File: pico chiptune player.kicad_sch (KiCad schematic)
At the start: 35 parts, among them J2 MicroSD, SW1 Play / Pause, SW2 Next, SW3 Previous, U1 AY-3-8910, U2 0.96"OLED_I2C, U3 PAM8302, U4 YM2149F, U5 PAM8302

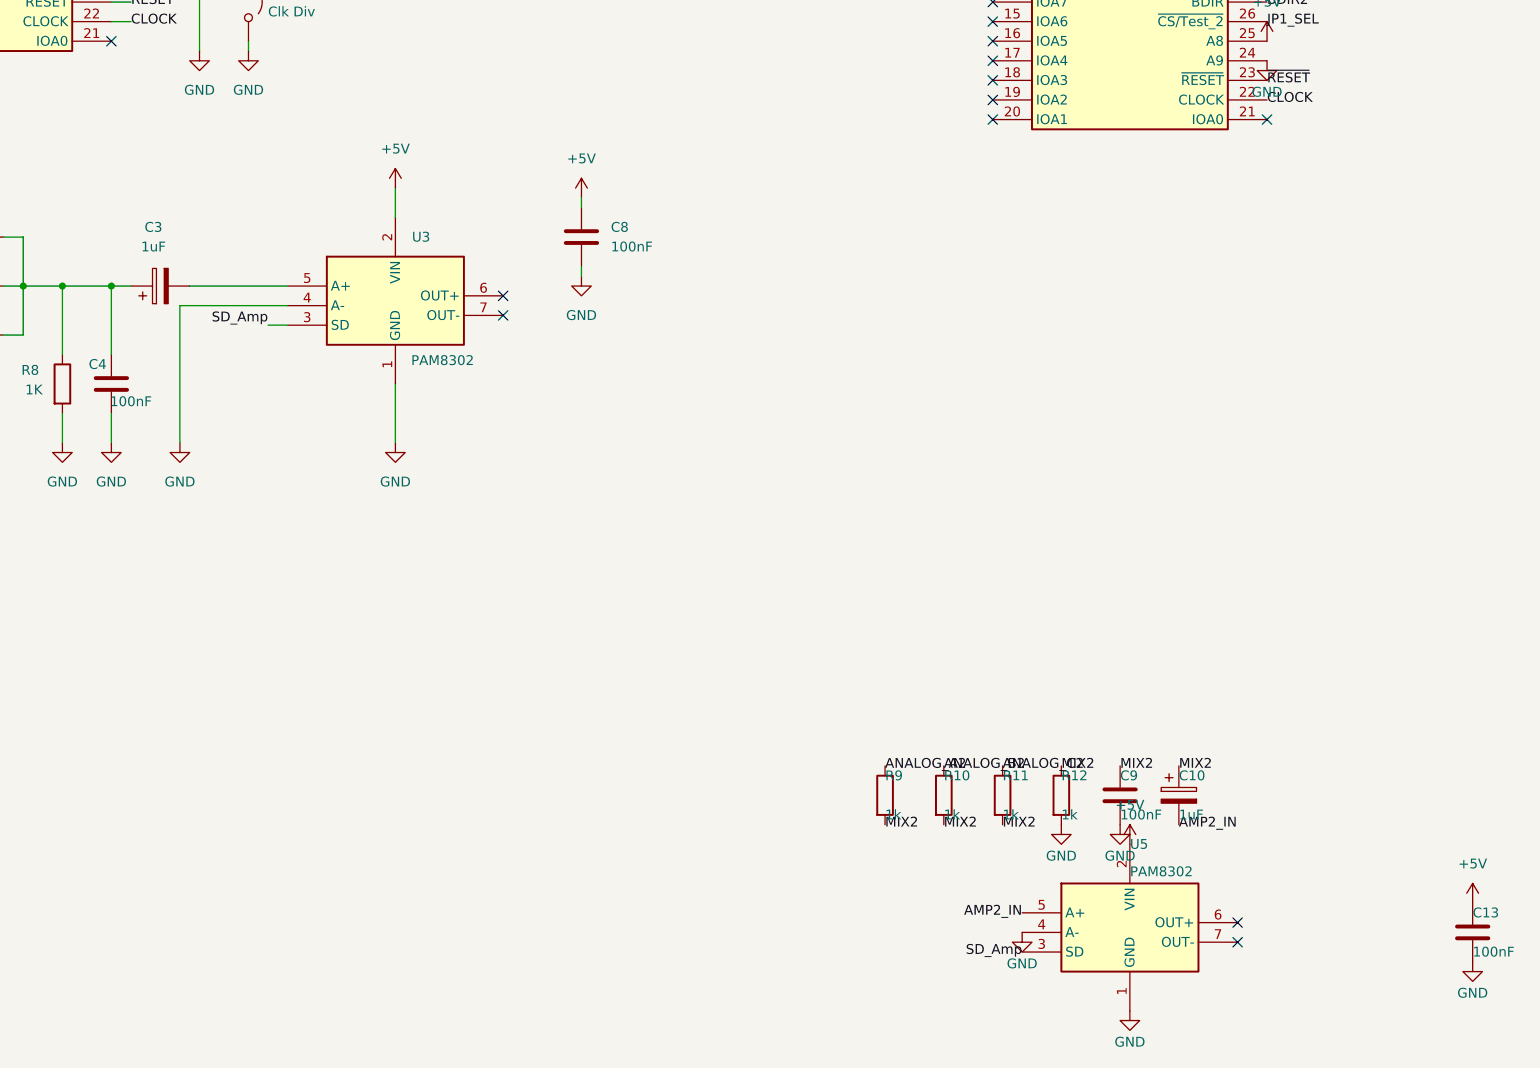
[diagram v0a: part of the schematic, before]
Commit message: Refactor code structure for improved readability and maintainability
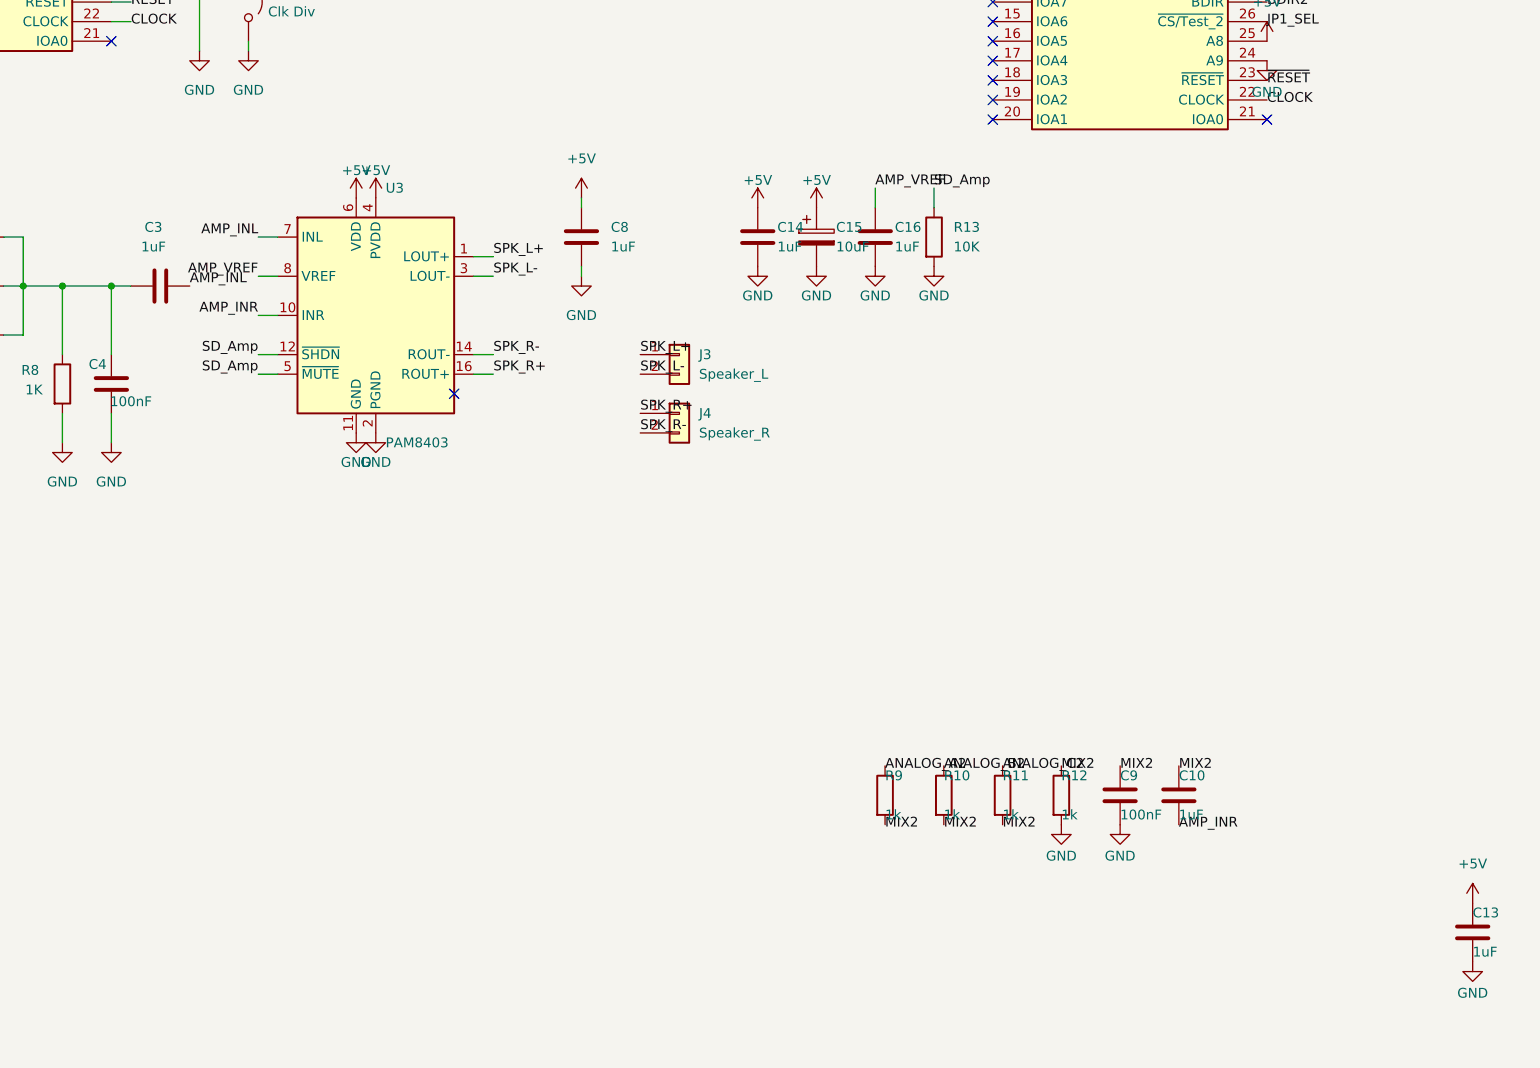
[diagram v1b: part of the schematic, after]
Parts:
- removed U3, U5: PAM8302, TModules:PAM8302A_Module, symbol terence:PAM8302
- added C14, C16: 1uF, Capacitor_SMD:C_0805_2012Metric_Pad1.18x1.45mm_HandSolder, symbol Device:C
- added C15: 10uF, Capacitor_SMD:CP_Elec_4x5.4, symbol Device:C_Polarized
- added J3: Speaker_L, Connector_JST:JST_PH_B2B-PH-K_1x02_P2.00mm_Vertical, symbol Connector_Generic:Conn_01x02
- added J4: Speaker_R, Connector_JST:JST_PH_B2B-PH-K_1x02_P2.00mm_Vertical, symbol Connector_Generic:Conn_01x02
- added R13: 10K, Resistor_SMD:R_0805_2012Metric_Pad1.20x1.40mm_HandSolder, symbol Device:R
- added U3: PAM8403, Package_SO:SOIC-16_3.9x9.9mm_P1.27mm, symbol Amplifier_Audio:PAM8403D
- C10: footprint Capacitor_SMD:CP_Elec_3x5.4 -> Capacitor_SMD:C_0805_2012Metric_Pad1.18x1.45mm_HandSolder; symbol Device:C_Polarized -> Device:C; LCSC Part # (none) -> C28323
- C13: value 100nF -> 1uF; LCSC Part # (none) -> C28323
- C3: footprint Capacitor_SMD:CP_Elec_3x5.4 -> Capacitor_SMD:C_0805_2012Metric_Pad1.18x1.45mm_HandSolder; symbol Device:C_Polarized -> Device:C; LCSC Part # C3348 -> C28323
- C8: value 100nF -> 1uF; LCSC Part # C1710 -> C28323
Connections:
- net +5V: now also C14.1, C15.1, U3.13 (PVDD), U3.4 (PVDD), U3.6 (VDD)
- net GND: now also C14.2, C15.2, C16.2, R13.2, U3.11 (GND), U3.15 (PGND), U3.2 (PGND)
- net SD_Amp: now also R13.1, U3.12 (~{SHDN}), U3.5 (~{MUTE})
- net AMP_INL: now reaches C3.2
- net AMP_INL: now also U3.7 (INL)
- net AMP2_IN renamed AMP_INR
- net AMP_INR: now also U3.10 (INR)
- new net AMP_VREF: C16.1, U3.8 (VREF)
- new net SPK_L+: J3.1 (Pin_1), U3.1 (LOUT+)
- new net SPK_L-: J3.2 (Pin_2), U3.3 (LOUT-)
- new net SPK_R+: J4.1 (Pin_1), U3.16 (ROUT+)
- new net SPK_R-: J4.2 (Pin_2), U3.14 (ROUT-)
- no-connect marks 47 -> 44
